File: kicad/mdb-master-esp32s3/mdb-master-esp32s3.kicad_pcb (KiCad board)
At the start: 2 copper layers, 41.8 x 50.2 mm, 40 parts, among them J2 MDB_Connector, J3 Barrel_Jack, J5 Conn_02x10_Odd_Even, P1 USB_C_Plug_USB2.0, Q1 BC807, U2 LM317_SOT-223, Y1 Crystal

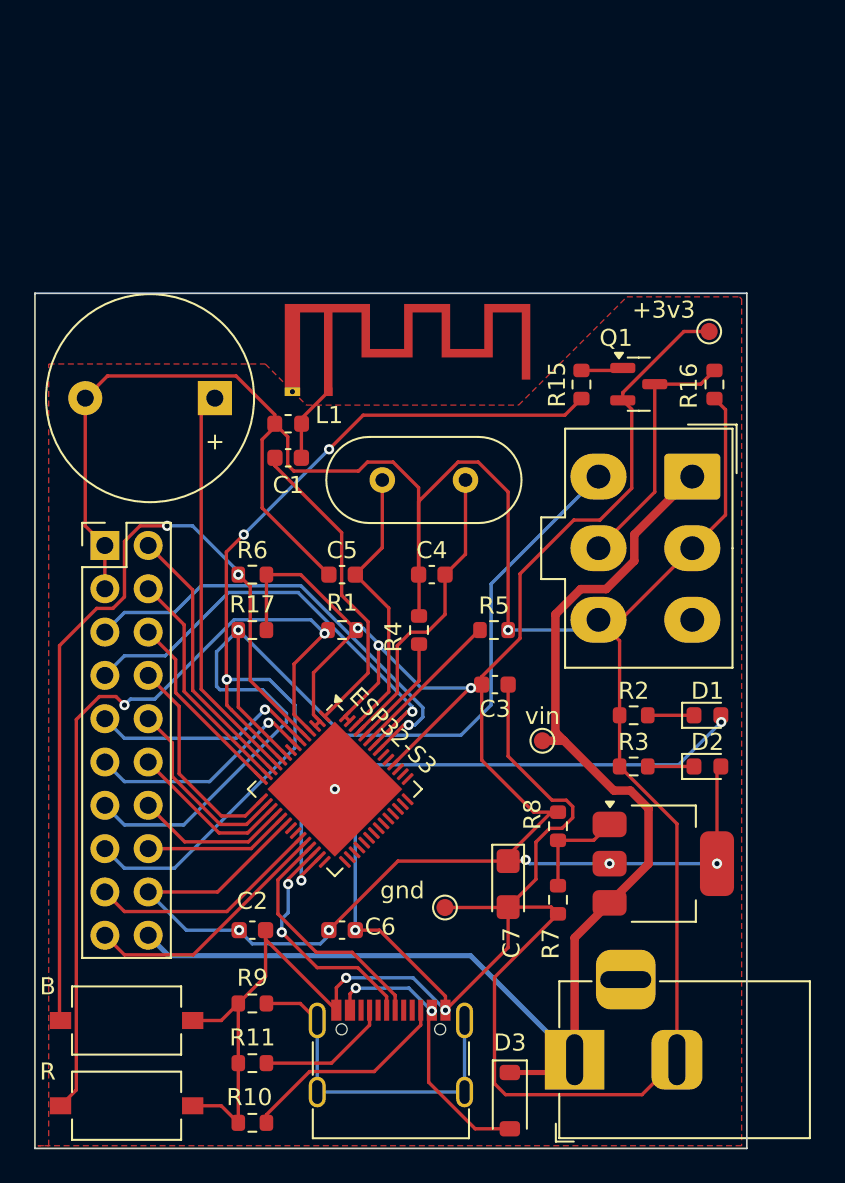
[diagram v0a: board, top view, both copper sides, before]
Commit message: Refacting kicad pcb
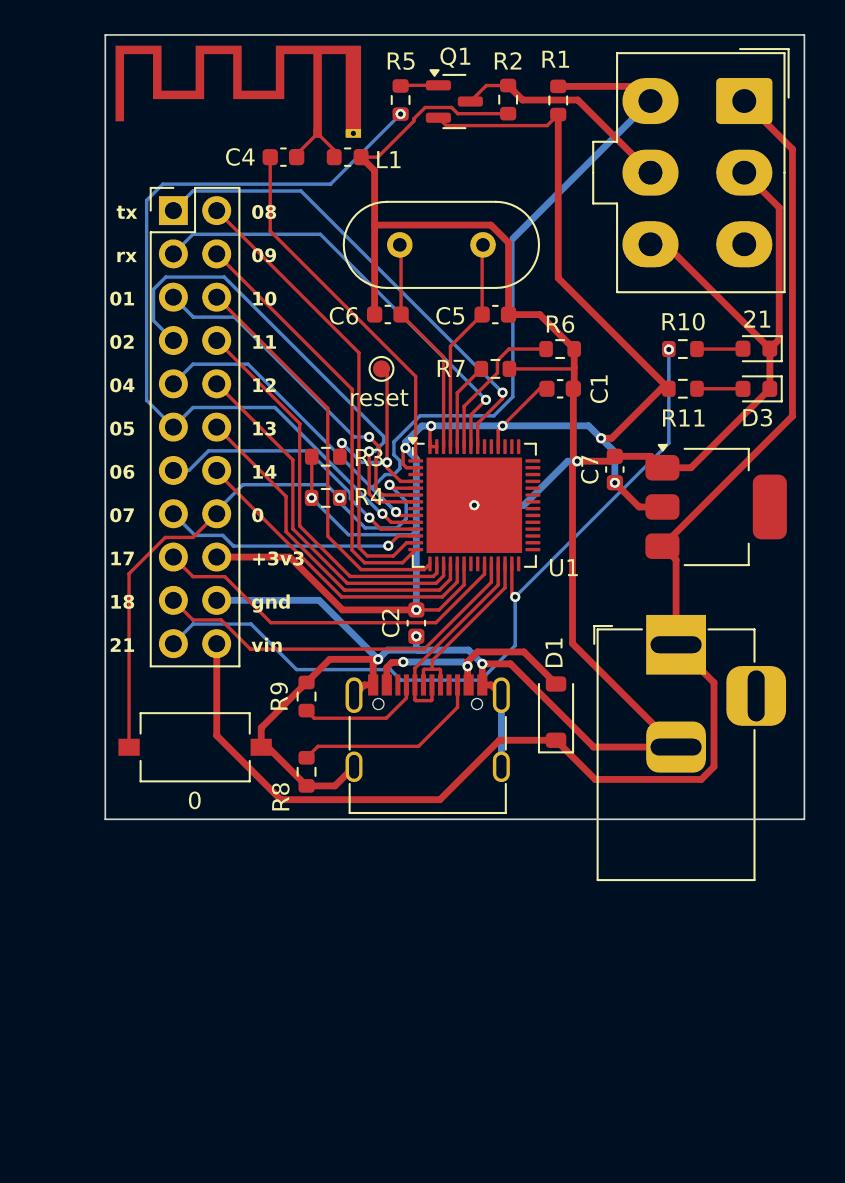
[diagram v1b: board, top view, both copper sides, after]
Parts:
- removed +3v3, gnd, vin: TestPoint, TestPoint:TestPoint_Pad_D1.0mm
- removed B: Boot, Button_Switch_SMD:SW_Tactile_SPST_NO_Straight_CK_PTS636Sx25SMTRLFS
- removed BZ1: Buzzer, Buzzer_Beeper:Buzzer_12x9.5RM7.6
- removed C3: C, Capacitor_SMD:C_0603_1608Metric
- removed D2: LED, LED_SMD:LED_0603_1608Metric
- removed ESP32-S3: ESP32-S3, Package_DFN_QFN:QFN-56-1EP_7x7mm_P0.4mm_EP5.6x5.6mm
- removed J5: Conn_02x10_Odd_Even, Connector_PinHeader_2.54mm:PinHeader_2x10_P2.54mm_Vertical
- removed P1: USB_C_Plug_USB2.0, Connector_USB:USB_C_Receptacle_G-Switch_GT-USB-7010ASV
- removed R: Reset, Button_Switch_SMD:SW_Tactile_SPST_NO_Straight_CK_PTS636Sx25SMTRLFS
- removed R15, R16, R17: R, Resistor_SMD:R_0603_1608Metric
- added 0: SW_Push, Button_Switch_SMD:SW_Tactile_SPST_NO_Straight_CK_PTS636Sx25SMTRLFS, F.Cu at (131.1, 117.5)
- added 21: LED, LED_SMD:LED_0603_1608Metric, F.Cu at (164.1, 94.1)
- added J1: MDB_Connector, Connector_Molex:Molex_Mini-Fit_Jr_5566-06A_2x03_P4.20mm_Vertical, F.Cu at (163.3, 79.6)
- added J4: Conn_02x11_Odd_Even, Connector_PinHeader_2.54mm:PinHeader_2x11_P2.54mm_Vertical, F.Cu at (129.9, 86.0)
- added U1: ESP32-S3R8, Package_DFN_QFN:QFN-56-1EP_7x7mm_P0.4mm_EP5.6x5.6mm, F.Cu at (147.5, 103.3)
- added reset: TestPoint, TestPoint:TestPoint_Pad_D1.0mm, F.Cu at (142.1, 95.3)
- AE1: footprint RF_Antenna:Texas_SWRA117D_2.4GHz_Right -> RF_Antenna:Texas_SWRA117D_2.4GHz_Left
- C4: value C -> 1.8pf
- C5, C6: value C -> 22pf
- C7: value C_Polarized -> 22pf; footprint Capacitor_Tantalum_SMD:CP_EIA-3216-18_Kemet-A -> Capacitor_SMD:C_0603_1608Metric
- D1: value LED -> 1N5819HWQ; footprint LED_SMD:LED_0603_1608Metric -> Diode_SMD:D_SOD-123
- D3: value D -> LED; footprint Diode_SMD:D_SOD-123 -> LED_SMD:LED_0603_1608Metric
- J2: value MDB_Connector -> Barrel_Jack; footprint Connector_Molex:Molex_Mini-Fit_Jr_5566-06A_2x03_P4.20mm_Vertical -> Connector_BarrelJack:BarrelJack_Horizontal
- J3: value Barrel_Jack -> USB_C_Receptacle_USB2.0_16P; footprint Connector_BarrelJack:BarrelJack_Horizontal -> Connector_USB:USB_C_Receptacle_G-Switch_GT-USB-7010ASV
- L1: value 47nH -> 2.4nh
- R1, R3, R4, R5, R6, R7, R9: value R -> 3.3k
- R10, R11: value R -> 240ohm
- R2: value R -> 180ohm
- R8: value 240 -> 3.3k
- U2: value LM317_SOT-223 -> AMS1117-3.3; footprint Package_TO_SOT_SMD:SOT-223-3_TabPin2 -> Package_TO_SOT_SMD:SOT-223
- Y1: value Crystal -> 40000hz
- moved R10 51.9 mm to (159.8, 94.1)
- moved R11 46.9 mm to (159.8, 96.5)
- moved D3 44.2 mm to (164.1, 96.5), turned to 180 degrees
- moved R2 36.9 mm to (149.5, 79.5), turned to -90 degrees
- moved C6 36.2 mm to (142.4, 92.1), turned to 0 degrees
- moved R1 33.5 mm to (152.4, 79.5), turned to 90 degrees
- moved R5 31.6 mm to (143.2, 79.5), turned to 90 degrees
- moved R7 31.4 mm to (148.8, 95.3), turned to 0 degrees
- moved C4 26.0 mm to (136.3, 82.9), turned to 180 degrees
- moved R3 25.6 mm to (138.8, 100.4)
- moved C7 25.1 mm to (155.8, 101.2)
- moved R6 22.4 mm to (152.6, 94.1)
- moved U2 21.1 mm to (161.7, 103.4)
- moved C2 20.4 mm to (144.1, 110.2), turned to -90 degrees
- moved J3 20.2 mm to (144.8, 117.5), turned to 0 degrees
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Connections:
- C1 pad 1: Net-(AE1-A) -> GND
- C1 pad 2: Net-(U1-LNA_IN/RF) -> +3V3
- C2 pad 1: GND -> +3V3
- C2 pad 2: +3V3 -> GND
- C4 pad 1: GND -> Net-(AE1-A)
- C4 pad 2: Net-(U1-XTAL_N) -> Net-(U1-LNA_IN/RF)
- C5 pad 2: Net-(U1-XTAL_P) -> Net-(U1-XTAL_N)
- C6 pad 2: +3V3 -> Net-(U1-XTAL_P)
- C7 pad 1: +3V3 -> GND
- C7 pad 2: GND -> +3V3
- D1 pad 1: Net-(D1-K) -> /vin
- D1 pad 2: /io21 -> Net-(D1-A)
- D3 pad 1: /vin -> GND
- J2 pad 3: unconnected-(J2-Pin_3-Pad3) -> (no net)
- L1 pad 1: Net-(AE1-A) -> GND
- L1 pad 2: GND -> Net-(AE1-A)
- R1 pad 2: Net-(U1-CHIP_PU/RESET) (its old number) -> /io4
- R10 pad 2: GND -> /io21
- R11 pad 1: Net-(P1-CC) -> Net-(D3-A)
- R11 pad 2: GND -> +3V3
- R2 pad 1: GND -> /mdb_master_transmit
- R2 pad 2: Net-(D1-K) -> GND
- R3 pad 1: GND -> +3V3
- R4 pad 1: Net-(U1-GPIO46) -> /boot
- R4 pad 2: GND -> +3V3
- R5 pad 1: Net-(U1-GPIO45) -> /io5
- R5 pad 2: GND -> Net-(Q1-B)
- R6 pad 1: /boot -> Net-(U1-GPIO45)
- R6 pad 2: +3V3 -> GND
- R7 pad 1: Net-(U2-ADJ) -> Net-(U1-GPIO46)
- R8 pad 1: +3V3 -> Net-(J3-CC2)
- R8 pad 2: Net-(U2-ADJ) -> GND
- R9 pad 1: Net-(P1-SHIELD) -> Net-(J3-CC1)
- U2 pad 1: Net-(U2-ADJ) -> GND
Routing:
- net GND: track 230.0 -> 170.5 mm
- net Net-(U1-CHIP_PU/RESET) (its old number): track 47.9 -> 0.00 mm, vias 2 -> 0
- net +3V3: track 133.5 -> 95.9 mm, vias 8 -> 7
- net Net-(P1-SHIELD): track 20.4 -> 0.00 mm
- net /boot: track 49.7 -> 34.1 mm
- net /io2: track 13.7 -> 28.0 mm
- net Net-(D3-A): track 16.6 -> 2.70 mm, vias 2 -> 0
- net /io9: track 11.4 -> 25.0 mm
- net Net-(D1-A): track 0.00 -> 13.6 mm, vias 0 -> 2
- net /io8: track 13.8 -> 27.1 mm
- net /io21: track 33.4 -> 45.9 mm
- net /io12: track 9.55 -> 21.4 mm
- net /io11: track 11.2 -> 22.8 mm
- net Net-(J3-CC2): track 0.00 -> 11.4 mm
- net /io5: track 59.7 -> 48.4 mm, vias 3 -> 2
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- removed copper zone on F.Cu, net GND
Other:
- board size 41.8 x 50.2 mm -> 41 x 46 mm
- board text added: "+3v3"
- board text added: "0"
- board text added: "01"
- board text added: "02"
- board text added: "04"
- board text added: "05"
- board text added: "06"
- board text added: "07"
- board text added: "08"
- board text added: "09"
- board text added: "10"
- board text added: "11"
- board text added: "12"
- board text added: "13"
- board text added: "14"
- board text added: "17"
- board text added: "18"
- board text added: "21"
- board text added: "gnd"
- board text added: "rx"
- board text added: "tx"
- board text added: "vin"
- board text removed: "7 gnd 8 gnd 9 tx 10 rx 11 1 12 2 13 4 14 5 +3v3 17 vin 18"

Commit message: Refacting kicad pcb
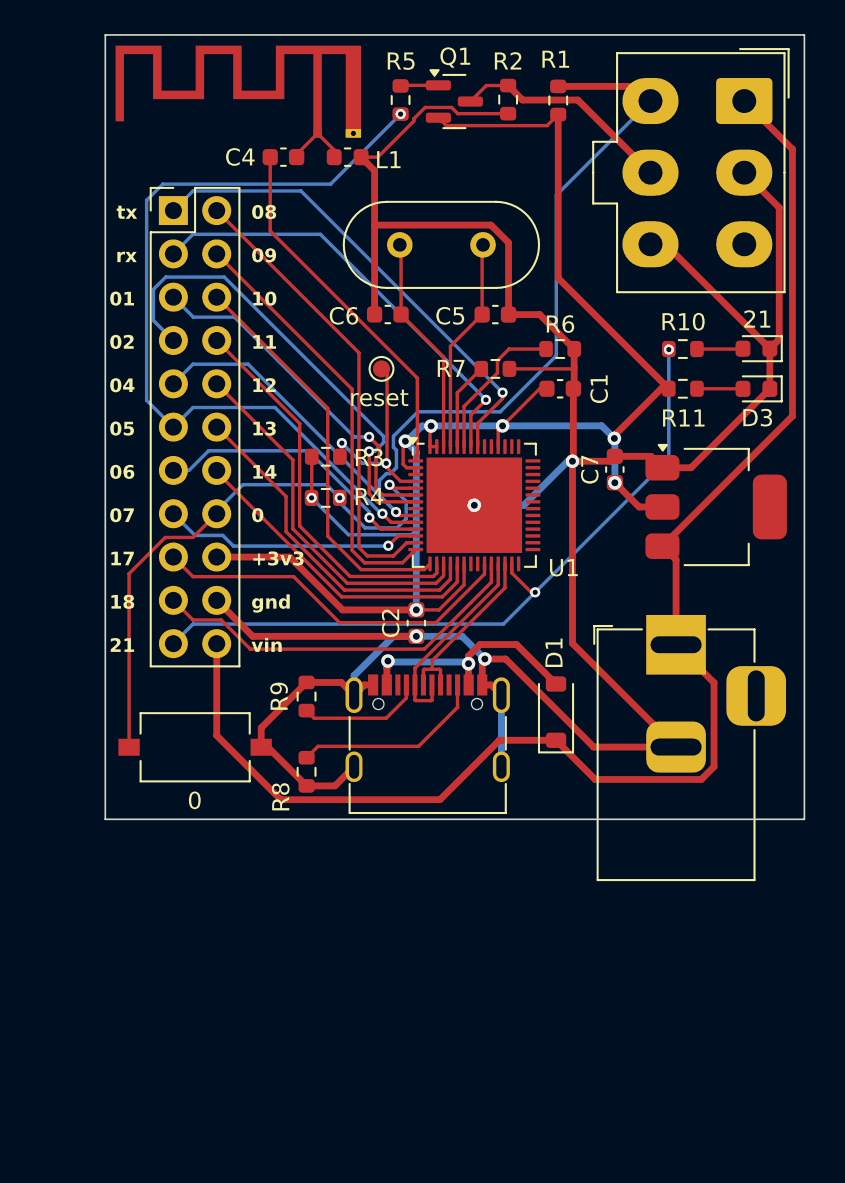
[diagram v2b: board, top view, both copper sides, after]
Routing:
- net /io21: track 45.9 -> 42.4 mm
- net GND: track 170.5 -> 171.5 mm, vias 5 -> 4
- net Net-(D1-A): track 13.6 -> 14.3 mm
